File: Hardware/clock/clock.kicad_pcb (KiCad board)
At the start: 2 copper layers, 127.5 x 48 mm, 19 parts, among them J1 Barrel_Jack_Switch, U1 WEMOS_C3_mini, U2 MAX7221xNG, U3 SBC18-11EGWA, U4 LM2596S-5, U5 SBC18-11EGWA, U6 SBC18-11EGWA, U7 SBC18-11EGWA

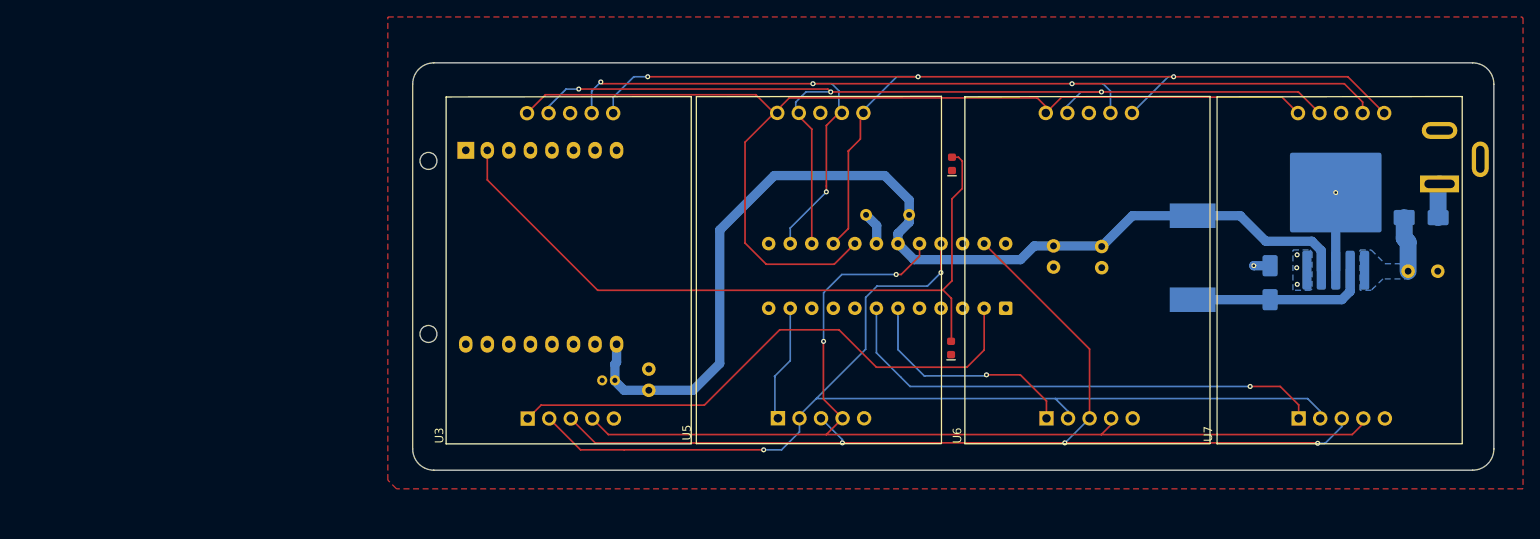
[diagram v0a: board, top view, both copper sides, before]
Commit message: Refactor code structure for improved readability and maintainability
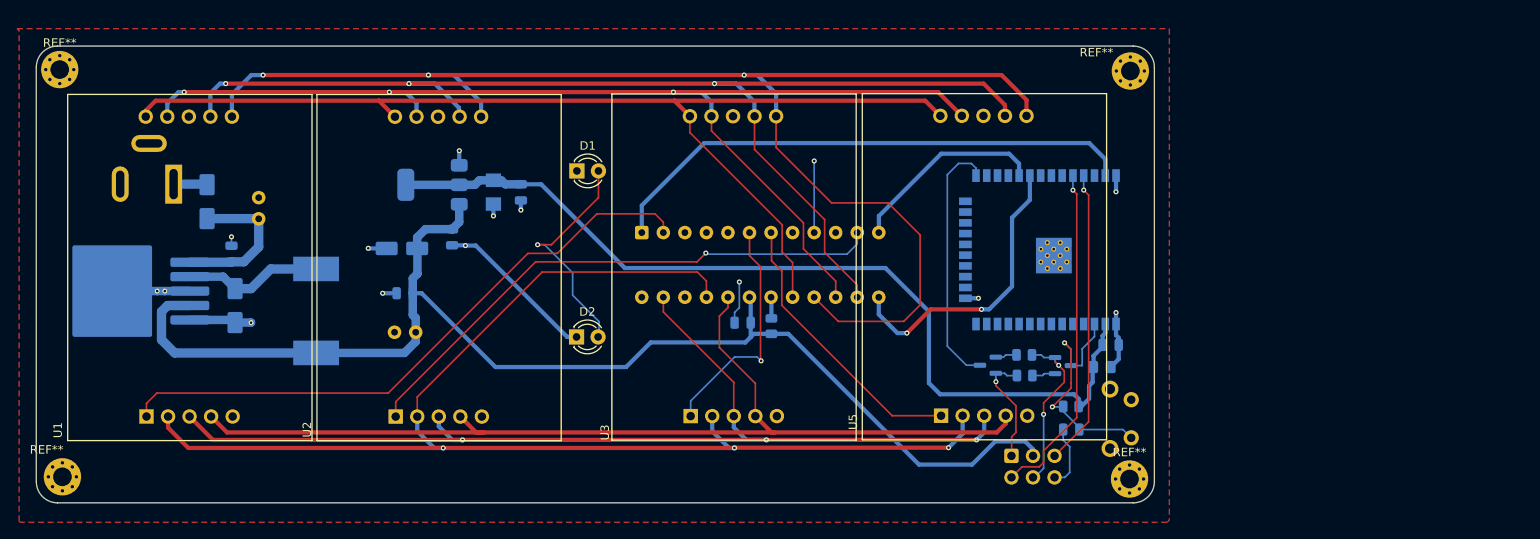
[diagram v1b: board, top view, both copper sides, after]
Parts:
- added C10: 100nF, SparkFun-Capacitor:C_0805_2012Metric, B.Cu at (85.8, 122.1)
- added C11: 100nF, SparkFun-Capacitor:C_0805_2012Metric, B.Cu at (164.4, 138.2)
- added C12: 100nF, SparkFun-Capacitor:C_0805_2012Metric, B.Cu at (125.6, 125.6)
- added C6: 100nF, SparkFun-Capacitor:C_0805_2012Metric, B.Cu at (99.5, 110.2)
- added C7: 22uF, Capacitor_SMD:C_0805_2012Metric_Pad1.18x1.45mm_HandSolder, B.Cu at (168.0, 130.8)
- added C8: 100nF, SparkFun-Capacitor:C_0805_2012Metric, B.Cu at (169.0, 128.2)
- added C9: 220uF, Capacitor_THT:C_Radial_D6.3mm_H5.0mm_P2.50mm, B.Cu at (87.1, 126.7)
- added J2: Conn_02x03_Top_Bottom, Connector_IDC:IDC-Header_2x03_P2.54mm_Horizontal, B.Cu at (157.3, 141.3)
- added Q1: BC817, Package_TO_SOT_SMD:SOT-23, B.Cu at (163.4, 130.6)
- added Q2: BC817, Package_TO_SOT_SMD:SOT-23, B.Cu at (154.6, 130.6)
- added R2: 10kΩ, PCM_JLCPCB:R_0805, B.Cu at (158.8, 129.4)
- added R3: 10kΩ, PCM_JLCPCB:R_0805, B.Cu at (158.9, 131.8)
- added R4: 10kΩ, PCM_JLCPCB:R_0805, B.Cu at (164.3, 135.4)
- added REF**: MountingHole_2.2mm_M2_Pad_Via, MountingHole:MountingHole_2.2mm_M2_Pad_Via, F.Cu at (171.2, 144.0)
- added REF**: MountingHole_2.2mm_M2_Pad_Via, MountingHole:MountingHole_2.2mm_M2_Pad_Via, F.Cu at (45.1, 95.7)
- added REF**: MountingHole_2.2mm_M2_Pad_Via, MountingHole:MountingHole_2.2mm_M2_Pad_Via, F.Cu at (171.3, 95.9)
- added REF**: MountingHole_2.2mm_M2_Pad_Via, MountingHole:MountingHole_2.2mm_M2_Pad_Via, F.Cu at (45.5, 143.7)
- added SW1: PTH_RA_h7.5mm, SparkFun-Switch:Push_PTH_RA_8-020_h7.5mm, B.Cu at (171.4, 136.9)
- added U8: LM2596S-5, Package_TO_SOT_SMD:TO-263-5_TabPin3, B.Cu at (52.8, 121.8)
- C1: value 680uF -> 10uF; footprint Capacitor_THT:C_Radial_D8.0mm_H11.5mm_P3.50mm -> Capacitor_SMD:CP_Elec_4x5.4
- C2: value 220uF -> 100nF; footprint Capacitor_THT:C_Radial_D6.3mm_H5.0mm_P2.50mm -> SparkFun-Capacitor:C_0805_2012Metric
- C3: value 104 -> 680uF; footprint Capacitor_THT:C_Disc_D3.0mm_W1.6mm_P2.50mm -> Capacitor_THT:C_Radial_D6.3mm_H7.0mm_P2.50mm
- C4: value 1uF -> 100nF; footprint Capacitor_THT:C_Radial_D4.0mm_H5.0mm_P1.50mm -> SparkFun-Capacitor:C_0805_2012Metric
- C5: value 104 -> 22uF; footprint Capacitor_THT:C_Disc_D3.0mm_W1.6mm_P2.50mm -> SparkFun-Fuse:1206
- D1: value M7 -> Red; footprint PCM_JLCPCB:D_SMA -> LED_THT:LED_D3.0mm; moved to F.Cu
- D2: value SS24 -> Red; footprint PCM_JLCPCB:D_SMA -> LED_THT:LED_D3.0mm; moved to F.Cu
- D3: value Red -> SS34; footprint SparkFun-LED:LED_0603_1608Metric_Red -> Diode_SMD:D_SMA; moved to B.Cu
- D4: value Red -> SS24; footprint SparkFun-LED:LED_0603_1608Metric_Red -> PCM_JLCPCB:D_SMA; moved to B.Cu
- R1: value 10k -> 10kΩ; footprint Resistor_THT:R_Axial_DIN0204_L3.6mm_D1.6mm_P5.08mm_Horizontal -> PCM_JLCPCB:R_0805
- U1: value WEMOS_C3_mini -> SBC18-11EGWA; footprint RF_Module:WEMOS_C3_mini -> Display_7Segment:SBC18-11SURKCGKWA; moved to F.Cu
- U2: value MAX7221xNG -> SBC18-11EGWA; footprint Package_DIP:DIP-24_W7.62mm -> Display_7Segment:SBC18-11SURKCGKWA; moved to F.Cu
- U4: value LM2596S-5 -> ESP32-WROOM-32; footprint Package_TO_SOT_SMD:TO-263-5_TabPin3 -> RF_Module:ESP32-WROOM-32
- U6: value SBC18-11EGWA -> MAX7221xNG; footprint Display_7Segment:SBC18-11SURKCGKWA -> Package_DIP:DIP-24_W7.62mm; moved to B.Cu
- U7: value SBC18-11EGWA -> AMS1117-3.3; footprint Display_7Segment:SBC18-11SURKCGKWA -> Package_TO_SOT_SMD:SOT-223-3_TabPin2; moved to B.Cu
- moved J1 149.2 mm to (58.6, 109.2), turned to 90 degrees
- moved C1 118.7 mm to (85.5, 116.8), turned to 180 degrees
- moved U7 109.9 mm to (89.1, 109.3), turned to 180 degrees
- moved L1 103.5 mm to (75.4, 124.2), turned to -90 degrees
- moved D1 99.7 mm to (106.1, 107.7)
- moved D3 87.9 mm to (62.5, 111.3)
- moved D4 84.6 mm to (65.8, 123.6), turned to -90 degrees
- moved U2 82.8 mm to (75.4, 139.5)
- moved D2 82.0 mm to (106.1, 127.2), turned to 0 degrees
- moved C2 76.6 mm to (91.4, 115.5)
- moved C5 66.3 mm to (96.3, 110.2)
- moved U1 58.2 mm to (45.9, 139.5), turned to 90 degrees
- moved U6 56.6 mm to (113.8, 115.0), turned to -90 degrees
- moved C3 50.2 mm to (68.6, 113.3)
- moved C4 47.6 mm to (65.4, 117.4), turned to 90 degrees
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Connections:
- C1 pad 1: /pwr_in -> +5V
- C3 pad 1: +5V -> /pwr_in
- C4 pad 1: +5V -> /pwr_in
- C5 pad 1: +5V -> 3.3V
- D1 pad 1: /pwr_in -> GND
- D1 pad 2: Net-(D1-Pad2) -> /Sec
- D2 pad 1: Net-(U4-OUT) -> GND
- D2 pad 2: GND -> /Sec
- D3 pad 1: GND -> /pwr_in
- D3 pad 2: /Sec -> Net-(D3-A)
- D4 pad 1: GND -> Net-(U8-OUT)
- D4 pad 2: /Sec -> GND
- J1 pad 1: Net-(D1-Pad2) -> Net-(D3-A)
- L1 pad 1: Net-(U4-OUT) -> Net-(U8-OUT)
- R1 pad 1: +5V -> Net-(U6-ISET)
- R1 pad 2: Net-(U2-ISET) -> +5V
- U1 pad 1: unconnected-(U1-EN-Pad1) -> /DIG_0
- U1 pad 10: GND -> /G
- U1 pad 2: /Sec -> /E
- U1 pad 3: unconnected-(U1-D2-Pad3) -> /D
- U1 pad 4: unconnected-(U1-D1-Pad4) -> /C
- U1 pad 6: unconnected-(U1-D4-Pad6) -> /B
- U1 pad 7: unconnected-(U1-D5-Pad7) -> /A
- U1 pad 9: +5V -> /F
- U2 pad 1: unconnected-(U2-DIN-Pad1) -> /DIG_1
- U2 pad 10: unconnected-(U2-DIG_5-Pad10) -> /G
- U2 pad 2: /DIG_0 -> /E
- U2 pad 3: unconnected-(U2-DIG_4-Pad3) -> /D
- U2 pad 4: GND -> /C
- U2 pad 6: /DIG_2 -> /B
- U2 pad 7: /DIG_3 -> /A
- U2 pad 9: GND -> /F
- U3 pad 1: /DIG_0 -> /DIG_2
- U4 pad 1: /pwr_in -> GND
- U4 pad 2: Net-(U4-OUT) -> 3.3V
- U4 pad 3: GND -> /EN
- U4 pad 4: +5V -> unconnected-(U4-SENSOR_VP-Pad4)
- U4 pad 5: GND -> unconnected-(U4-SENSOR_VN-Pad5)
- U5 pad 1: /DIG_1 -> /DIG_3
- U6 pad 1: /DIG_2 -> /MOSI
- U6 pad 10: /G -> unconnected-(U6-DIG_5-Pad10)
- U6 pad 2: /E -> /DIG_0
- U6 pad 3: /D -> unconnected-(U6-DIG_4-Pad3)
- U6 pad 4: /C -> GND
- U6 pad 6: /B -> /DIG_2
- U6 pad 7: /A -> /DIG_3
- U6 pad 9: /F -> GND
- U7 pad 1: /DIG_3 -> GND
- U7 pad 2: /E -> 3.3V
- U7 pad 3: /D -> +5V
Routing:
- net 3.3V: track 0.00 -> 107.1 mm
- net GND: track 11.1 -> 76.0 mm, vias 5 -> 15
- net /MOSI: track 0.00 -> 63.6 mm
- net /Sec: track 86.5 -> 27.1 mm, vias 0 -> 1
- net /DIG_1: track 13.8 -> 65.3 mm, vias 0 -> 1
- net /RXD0: track 0.00 -> 40.1 mm, vias 0 -> 1
- net /B: track 127.5 -> 164.6 mm
- net /TXD0: track 0.00 -> 34.9 mm, vias 0 -> 1
- net /CLK: track 0.00 -> 34.9 mm, vias 0 -> 2
- net /EN: track 0.00 -> 30.2 mm, vias 0 -> 2
- net /IO0: track 0.00 -> 30.0 mm
- net +5V: track 123.2 -> 150.6 mm
- net /E: track 128.3 -> 154.4 mm, vias 2 -> 3
- net /DIG_3: track 59.2 -> 33.3 mm, vias 1 -> 0
- net /CS: track 0.00 -> 23.4 mm
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- removed copper zone on B.Cu, net /pwr_in
- removed copper zone on B.Cu, net GND
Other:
- board size 127.5 x 48 mm -> 131.8 x 53.9 mm
